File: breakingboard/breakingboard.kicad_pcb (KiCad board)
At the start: 2 copper layers, 13 parts, among them U2 STM32F103C8T6, Y1 16MHz

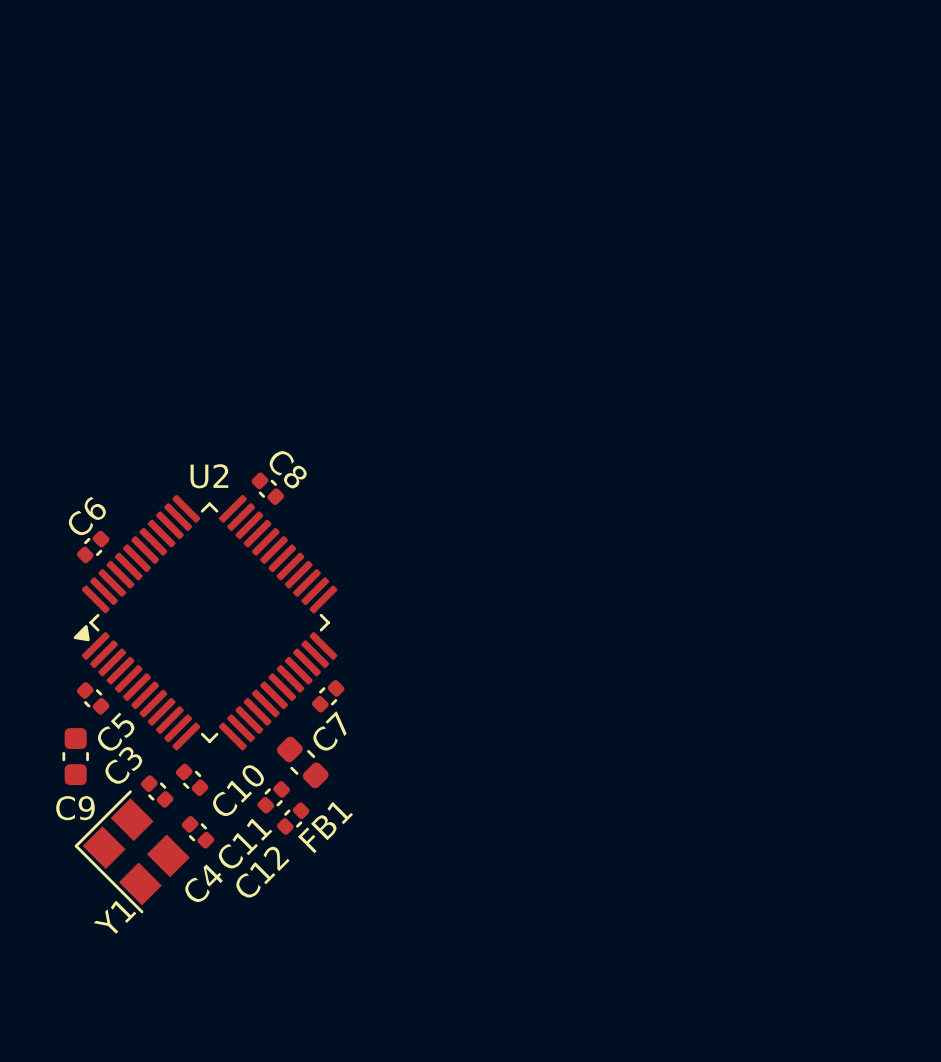
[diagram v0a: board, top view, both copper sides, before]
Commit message: pushing to save
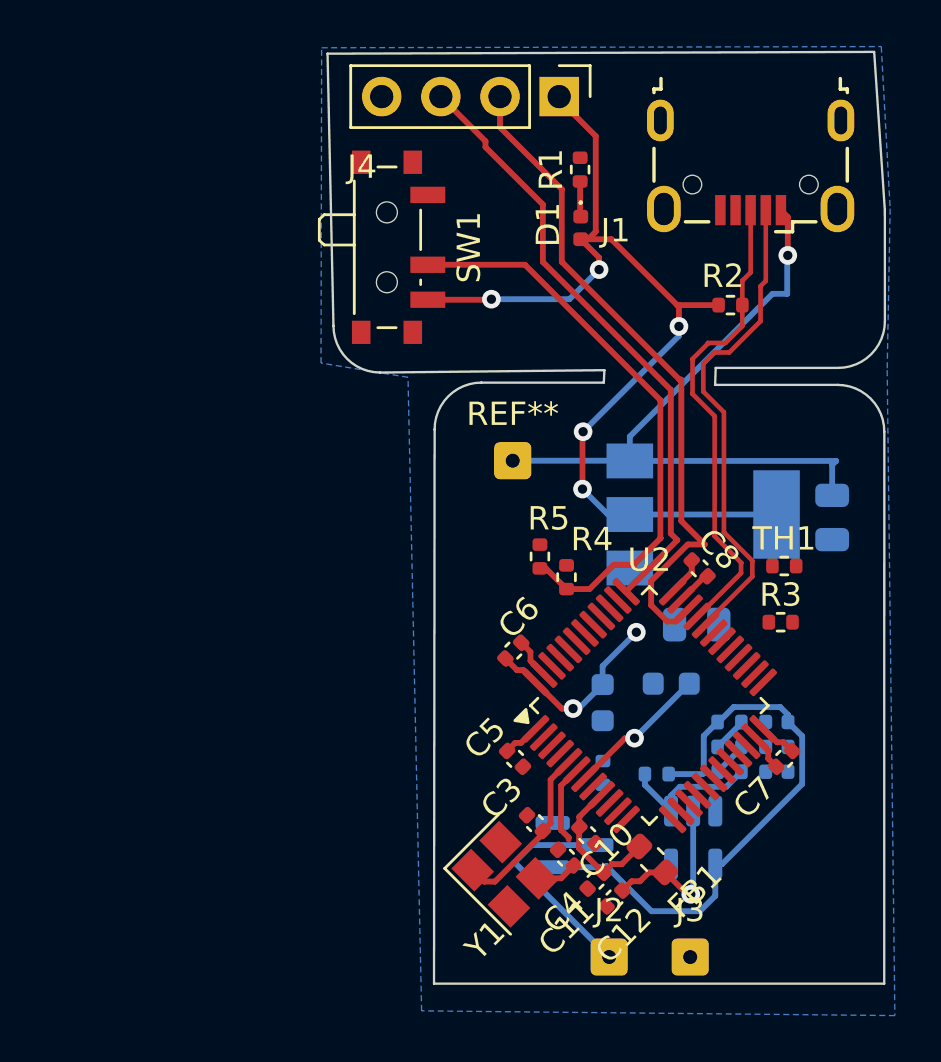
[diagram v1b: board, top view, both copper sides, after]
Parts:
- added C1: 22uF, Capacitor_SMD:C_0805_2012Metric, B.Cu at (58.0, 36.9)
- added C13: 10uF, Capacitor_SMD:C_0603_1608Metric, B.Cu at (51.1, 44.0)
- added C14: 0.015u, Capacitor_SMD:C_0402_1005Metric, B.Cu at (55.7, 47.8)
- added C15: 0.015u, Capacitor_SMD:C_0402_1005Metric, B.Cu at (55.7, 46.8)
- added C16: .015u, Capacitor_SMD:C_0402_1005Metric, B.Cu at (55.7, 45.7)
- added C2: 22uF, Capacitor_SMD:C_0805_2012Metric, B.Cu at (52.2, 41.5)
- added D1: LED, LED_SMD:LED_0402_1005Metric, F.Cu at (47.2, 24.5)
- added J1: USB_B_Micro, Connector_USB:USB_Micro-B_Wuerth_629105150521, F.Cu at (54.5, 21.8)
- added J2: MFC Connector Plus, Connector_Wire:SolderWire-0.1sqmm_1x01_D0.4mm_OD1mm, F.Cu at (48.5, 55.8)
- added J3: MFC Connector Minus, Connector_Wire:SolderWire-0.1sqmm_1x01_D0.4mm_OD1mm, F.Cu at (51.9, 55.8)
- added J4: Conn_01x04_Pin, Connector_PinHeader_2.54mm:PinHeader_1x04_P2.54mm_Vertical, F.Cu at (46.3, 18.8)
- added Q1: NPN, Package_TO_SOT_SMD:SOT-23, B.Cu at (47.0, 51.0)
- added R1: 1.5k, Resistor_SMD:R_0402_1005Metric, F.Cu at (47.2, 22.0)
- added R10: 1.5k, Resistor_SMD:R_0402_1005Metric, B.Cu at (48.2, 47.9)
- added R2: 1.5k, Resistor_SMD:R_0402_1005Metric, F.Cu at (53.7, 27.8)
- added R3: 4.7k, Resistor_SMD:R_0402_1005Metric, F.Cu at (55.8, 41.4)
- added R4: 10k, Resistor_SMD:R_0402_1005Metric, F.Cu at (46.6, 39.5)
- added R5: 1, Resistor_SMD:R_0402_1005Metric, F.Cu at (45.5, 38.6)
- added R6: 10k, Resistor_SMD:R_0402_1005Metric, B.Cu at (53.6, 47.8)
- added R7: 10k, Resistor_SMD:R_0402_1005Metric, B.Cu at (53.6, 46.8)
- added R8: 10k, Resistor_SMD:R_0402_1005Metric, B.Cu at (53.6, 45.7)
- added R9: 100Meg, Resistor_SMD:R_0402_1005Metric, B.Cu at (50.5, 47.9)
- added REF**: SolderWire-0.1sqmm_1x01_D0.4mm_OD1mm, Connector_Wire:SolderWire-0.1sqmm_1x01_D0.4mm_OD1mm, F.Cu at (44.3, 34.5)
- added SW1: SW_SPDT, Button_Switch_SMD:SW_SPDT_PCM12, F.Cu at (39.3, 25.3)
- added TH1: 100k, Resistor_SMD:R_0402_1005Metric, F.Cu at (56.0, 39.0)
- added U1: AMS1117-3.3, Package_TO_SOT_SMD:SOT-223-3_TabPin2, B.Cu at (52.5, 36.8)
- added U3: MCP6L01Rx-xOT, Package_TO_SOT_SMD:SOT-23-5, B.Cu at (52.1, 50.6)
- C9: moved to B.Cu
- moved C9 22.7 mm to (48.2, 44.9)
- moved C7 19.8 mm to (56.0, 47.3)
- moved U2 19.2 mm to (50.2, 45.0)
- moved C8 18.9 mm to (52.3, 39.1)
- moved C6 18.6 mm to (44.3, 42.6)
- moved C5 18.3 mm to (44.4, 47.3)
- moved C10 17.1 mm to (47.5, 50.5)
- moved C3 16.3 mm to (45.3, 50.0)
- moved Y1 15.9 mm to (44.0, 52.2)
- moved C4 15.8 mm to (46.6, 51.5)
- moved FB1 15.6 mm to (50.3, 51.6)
- moved C11 14.3 mm to (47.9, 52.5)
- moved C12 14.2 mm to (48.7, 53.3)
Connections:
- C12 pad 1: Net-(C12-Pad1) -> +3.3V
- FB1 pad 1: Net-(C12-Pad1) -> +3.3V
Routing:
- net +3.3V: track 0.00 -> 62.8 mm, vias 0 -> 8
- net VBUS: track 0.00 -> 29.5 mm, vias 0 -> 1
- net /SWDIO: track 0.00 -> 29.1 mm
- net /SWCLK: track 0.00 -> 26.4 mm
- net /MFC COM OUT: track 0.00 -> 25.2 mm
- net /sw_boot0: track 0.00 -> 24.8 mm
- net /USB_D-: track 0.00 -> 21.0 mm
- net /USB_D+: track 0.00 -> 20.6 mm
- net Net-(J2-Pin_1): track 0.00 -> 9.62 mm
- net /HSE_IN: track 0.00 -> 7.61 mm
- net +3.3VA: track 0.00 -> 6.19 mm
- net /NRESET: track 0.00 -> 6.16 mm, vias 0 -> 1
- net Net-(R6-Pad1): track 0.00 -> 6.16 mm
- net /HSE_OUT: track 0.00 -> 5.21 mm
- net GND: track 0.00 -> 4.97 mm
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- added copper zone on B.Cu, net GND
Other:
- board outline added: 23.9 x 40 mm
